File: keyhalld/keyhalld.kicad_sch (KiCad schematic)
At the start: 28 parts, among them J1 Conn_01x06_Pin, J2 Conn_01x04_Pin, SW1 RESET, SW2 USB_BOOT, U1 RP2350A, U2 CD74HC4067M, Y1 12MHz

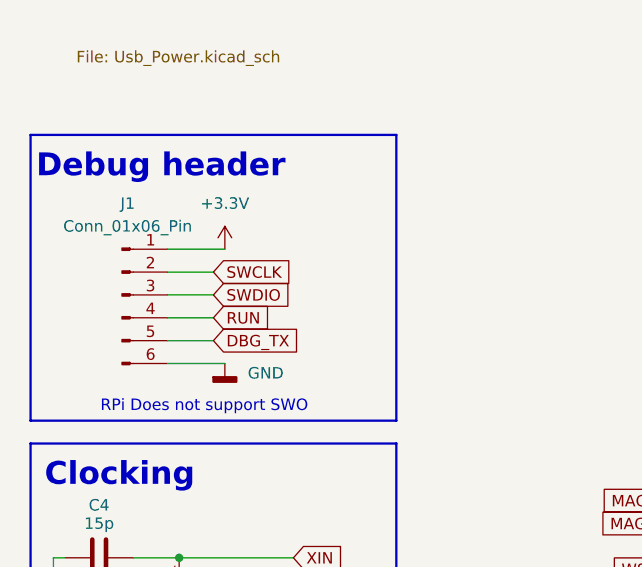
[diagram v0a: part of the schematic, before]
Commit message: Store WIP results
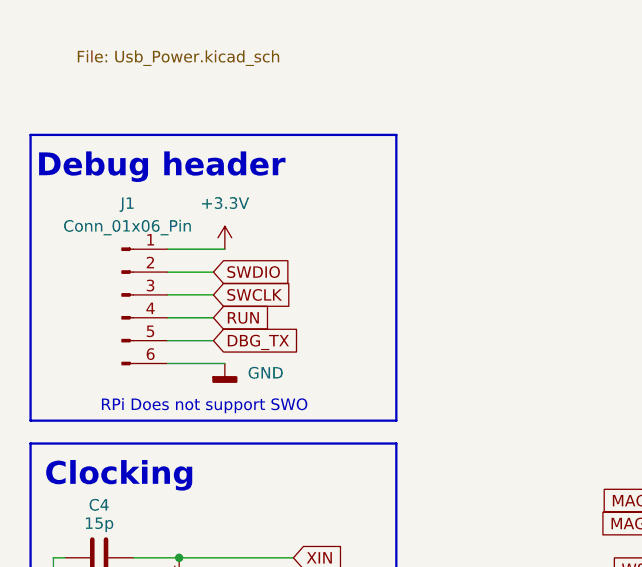
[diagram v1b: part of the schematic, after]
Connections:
- net SWCLK: now also J1.3 (Pin_3); no longer J1.2 (Pin_2)
- net SWDIO: now also J1.2 (Pin_2); no longer J1.3 (Pin_3)
